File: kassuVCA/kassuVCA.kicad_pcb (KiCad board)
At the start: 2 copper layers, 268 parts, among them J201 Conn_02x05_Odd_Even, Q1 MMBT3904, Q2 MMBT3904, Q3 MBT3904DW1, Q4 MBT3904DW1, Q401 MMBT3904, Q402 MBT3904DW1, Q403 MBT3904DW1, Q404 MMBT3904, Q5 MMBT3904, Q501 MMBT3904, Q502 MMBT3904, Q503 MBT3904DW1, Q504 MBT3904DW1, Q6 MMBT3904, Q7 MBT3904DW1, Q8 MBT3904DW1, U1 TL072, U2 TL072, U3 TL072, U301 TL074, U4 TL072, U401 TL072, U402 TL072, U501 TL072, U502 TL072

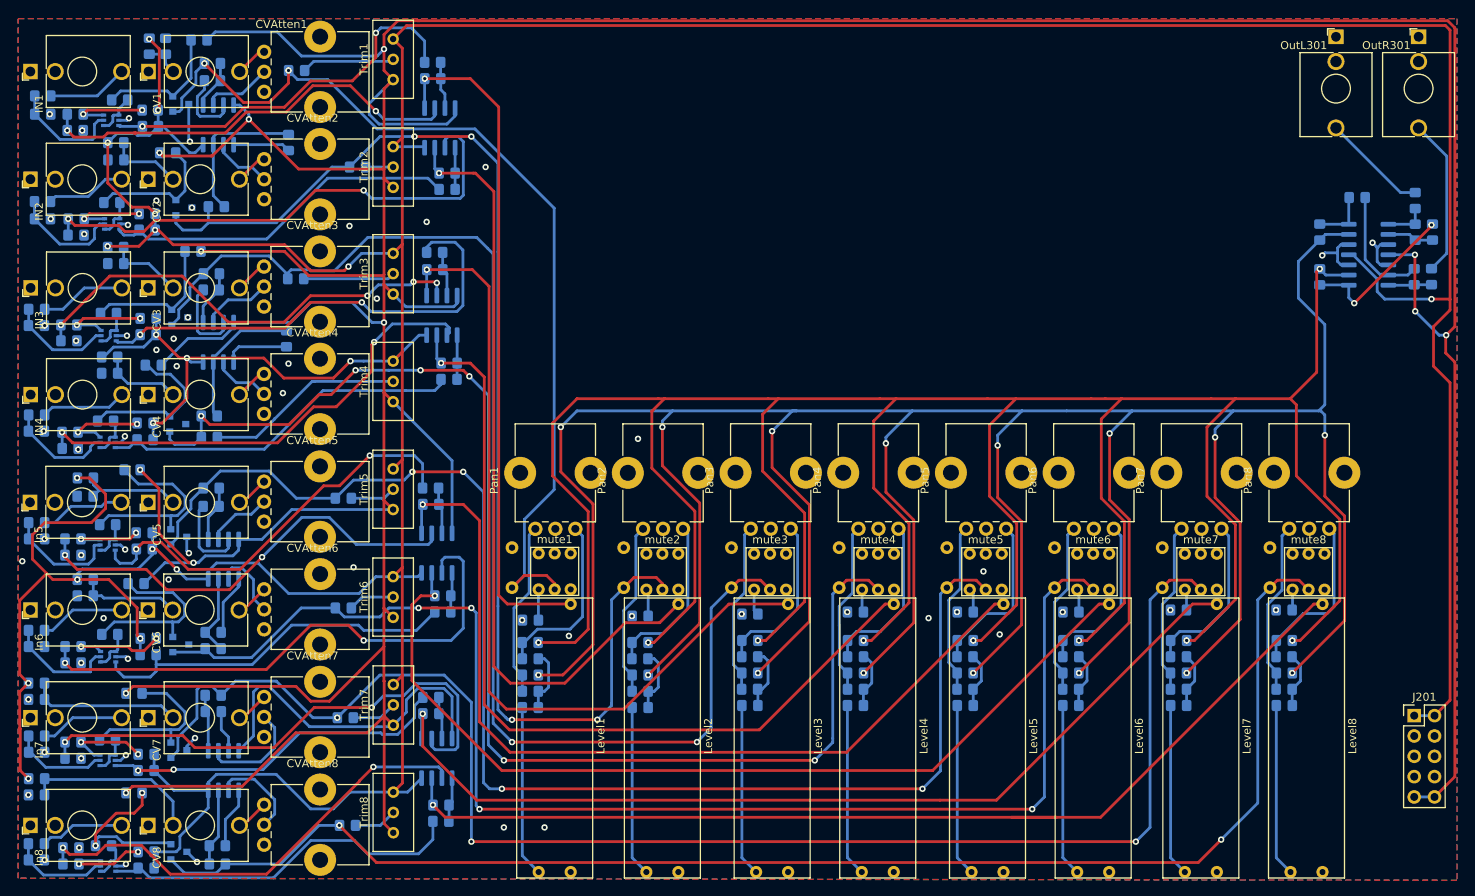
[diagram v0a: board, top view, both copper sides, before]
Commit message: bigMix
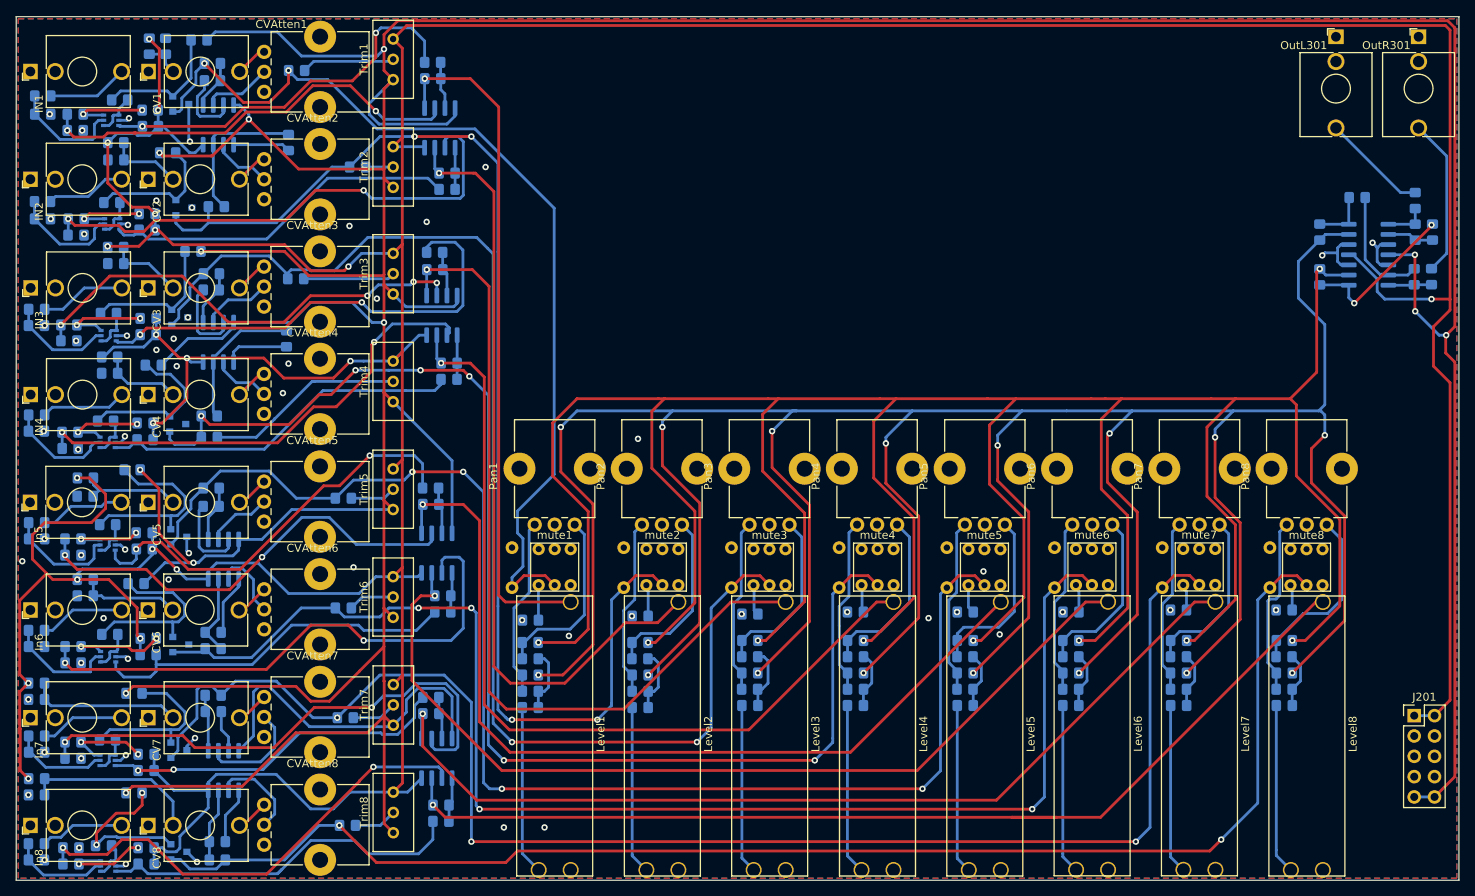
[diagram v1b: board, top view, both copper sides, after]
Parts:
- moved mute7 0.63 mm to (173.3, 94.2)
- moved mute8 0.61 mm to (186.7, 94.2)
- moved mute6 0.60 mm to (159.9, 94.2)
- moved Pan8 0.59 mm to (189.2, 88.9)
- moved mute5 0.58 mm to (146.4, 94.2)
- moved mute4 0.57 mm to (133.1, 94.2)
- moved mute2 0.57 mm to (106.2, 94.2)
- moved Pan7 0.56 mm to (175.8, 88.9)
- moved mute3 0.56 mm to (119.6, 94.2)
- moved Pan6 0.54 mm to (162.4, 88.9)
- moved Pan4 0.54 mm to (135.5, 88.9)
- moved Pan2 0.53 mm to (108.6, 88.9)
- moved mute1 0.53 mm to (92.7, 94.2)
- moved Pan5 0.53 mm to (149.0, 88.9)
- moved Pan1 0.53 mm to (95.2, 88.9)
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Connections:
- IN1 pad TN: (no net) -> unconnected-(IN1-PadTN)
- IN2 pad TN: (no net) -> unconnected-(IN2-PadTN)
- IN3 pad TN: (no net) -> unconnected-(IN3-PadTN)
- IN4 pad TN: (no net) -> unconnected-(IN4-PadTN)
- In5 pad TN: (no net) -> unconnected-(In5-PadTN)
- In6 pad TN: (no net) -> unconnected-(In6-PadTN)
- In7 pad TN: (no net) -> unconnected-(In7-PadTN)
- In8 pad TN: (no net) -> unconnected-(In8-PadTN)
- OutL301 pad TN: (no net) -> unconnected-(OutL301-PadTN)
- OutR301 pad TN: (no net) -> unconnected-(OutR301-PadTN)
- mute1 pad 3: (no net) -> unconnected-(mute1-Pad3)
- mute1 pad 4: (no net) -> unconnected-(mute1-Pad4)
- mute1 pad 5: (no net) -> unconnected-(mute1-Pad5)
- mute1 pad 6: (no net) -> unconnected-(mute1-Pad6)
- mute2 pad 3: (no net) -> unconnected-(mute2-Pad3)
- mute2 pad 4: (no net) -> unconnected-(mute2-Pad4)
- mute2 pad 5: (no net) -> unconnected-(mute2-Pad5)
- mute2 pad 6: (no net) -> unconnected-(mute2-Pad6)
- mute3 pad 3: (no net) -> unconnected-(mute3-Pad3)
- mute3 pad 4: (no net) -> unconnected-(mute3-Pad4)
- mute3 pad 5: (no net) -> unconnected-(mute3-Pad5)
- mute3 pad 6: (no net) -> unconnected-(mute3-Pad6)
- mute4 pad 3: (no net) -> unconnected-(mute4-Pad3)
- mute4 pad 4: (no net) -> unconnected-(mute4-Pad4)
- mute4 pad 5: (no net) -> unconnected-(mute4-Pad5)
- mute4 pad 6: (no net) -> unconnected-(mute4-Pad6)
- mute5 pad 3: (no net) -> unconnected-(mute5-Pad3)
- mute6 pad 3: (no net) -> unconnected-(mute6-Pad3)
- mute7 pad 3: (no net) -> unconnected-(mute7-Pad3)
- mute8 pad 3: (no net) -> unconnected-(mute8-Pad3)
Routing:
- net Level1R: track 426.2 -> 429.9 mm
- net Level1L: track 401.6 -> 404.2 mm
- net Net-(Pan5-Pad1): track 21.0 -> 22.8 mm
- net Net-(Pan2-Pad1): track 21.0 -> 22.5 mm
- net Net-(Pan8-Pad1): track 21.0 -> 22.5 mm
- net Net-(Pan4-Pad1): track 20.9 -> 22.1 mm
- net Net-(Pan3-Pad1): track 21.0 -> 22.0 mm
- net Net-(Pan8-Pad3): track 21.6 -> 22.5 mm
- net Net-(Pan6-Pad1): track 21.1 -> 21.9 mm
- net Net-(Pan1-Pad1): track 22.3 -> 23.0 mm
- net Net-(R58-Pad2): track 2.56 -> 3.25 mm
- net Net-(R14-Pad2): track 2.98 -> 3.60 mm
- net Net-(Pan7-Pad1): track 21.1 -> 21.7 mm
- net Net-(R70-Pad1): track 58.5 -> 59.0 mm
- net Net-(Q8-Pad6): track 45.9 -> 46.5 mm
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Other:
- board outline added: 180.3 x 107.9 mm
- net class Default removed
- board text added: "-12V Red Stripe"
